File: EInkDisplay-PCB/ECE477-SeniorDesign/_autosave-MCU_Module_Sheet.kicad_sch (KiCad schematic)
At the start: 25 parts, among them SW1 SW_Push_Dual_x2, U3 STM32L496ZGTxP, Y1 32.768kHz

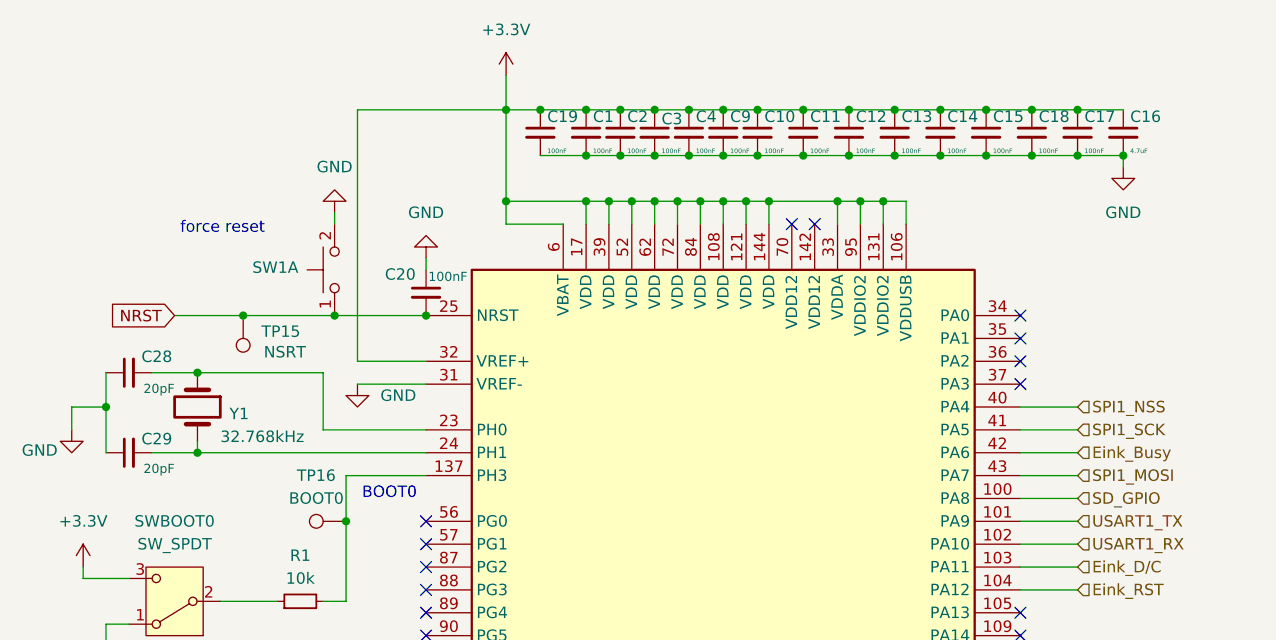
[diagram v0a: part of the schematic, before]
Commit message: changes
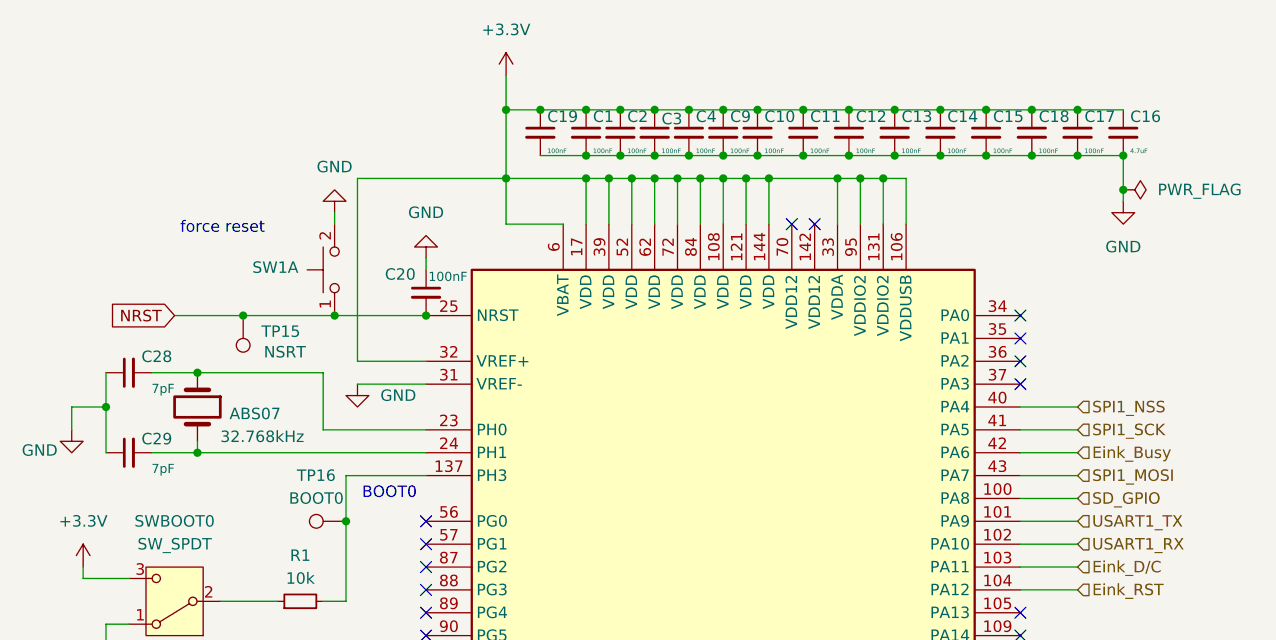
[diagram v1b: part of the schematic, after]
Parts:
- C1, C10, C11, C12, C13, C14, C15, C16, C17, C18, C19, C2, C3, C4, C9: footprint (none) -> Capacitor_SMD:C_0603_1608Metric_Pad1.08x0.95mm_HandSolder
- C28, C29: value 20pF -> 7pF; footprint (none) -> Capacitor_SMD:C_0603_1608Metric_Pad1.08x0.95mm_HandSolder
- renumbered Y1 to ABS07

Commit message: push
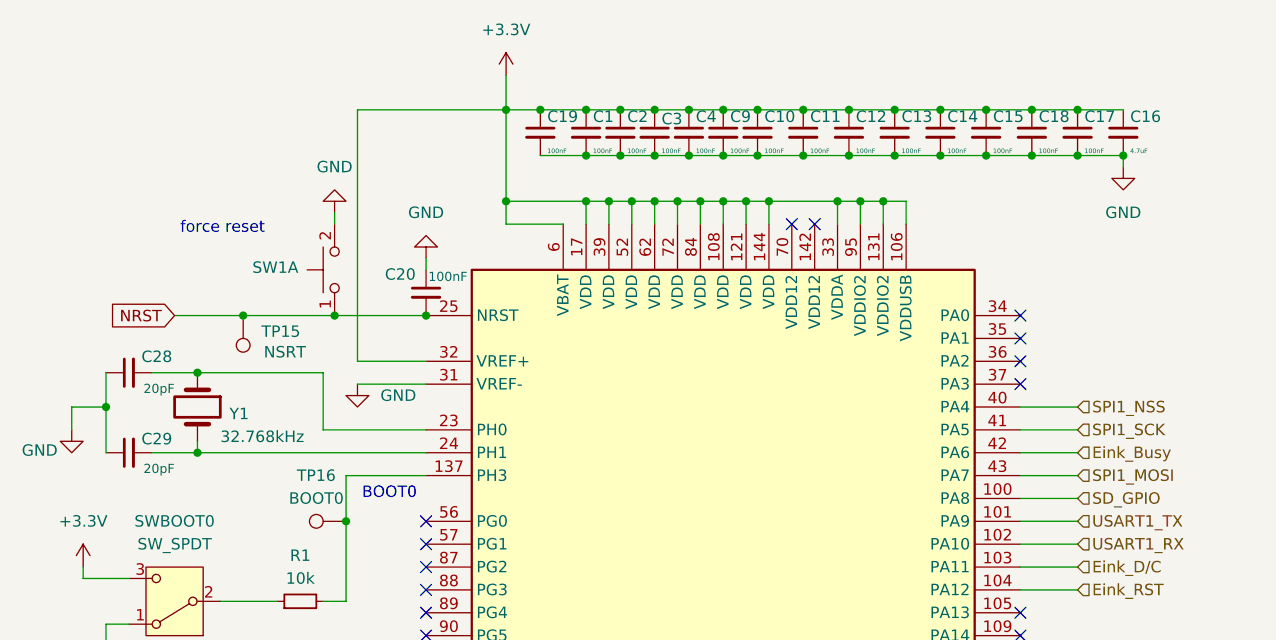
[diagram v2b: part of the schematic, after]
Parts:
- C1, C10, C11, C12, C13, C14, C15, C16, C17, C18, C19, C2, C3, C4, C9: footprint Capacitor_SMD:C_0603_1608Metric_Pad1.08x0.95mm_HandSolder -> (none)
- C28, C29: value 7pF -> 20pF; footprint Capacitor_SMD:C_0603_1608Metric_Pad1.08x0.95mm_HandSolder -> (none)
- renumbered ABS07 to Y1
